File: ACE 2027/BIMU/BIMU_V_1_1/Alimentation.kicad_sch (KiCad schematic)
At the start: 16 parts, among them U101 AP7361C-33E

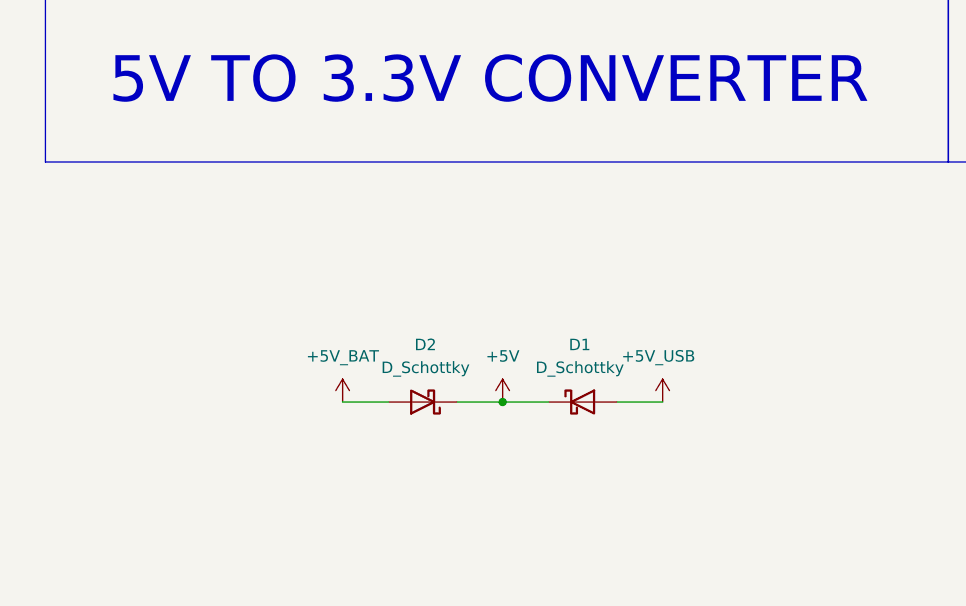
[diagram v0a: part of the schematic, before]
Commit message: Faire les modifications requise pour le pcb
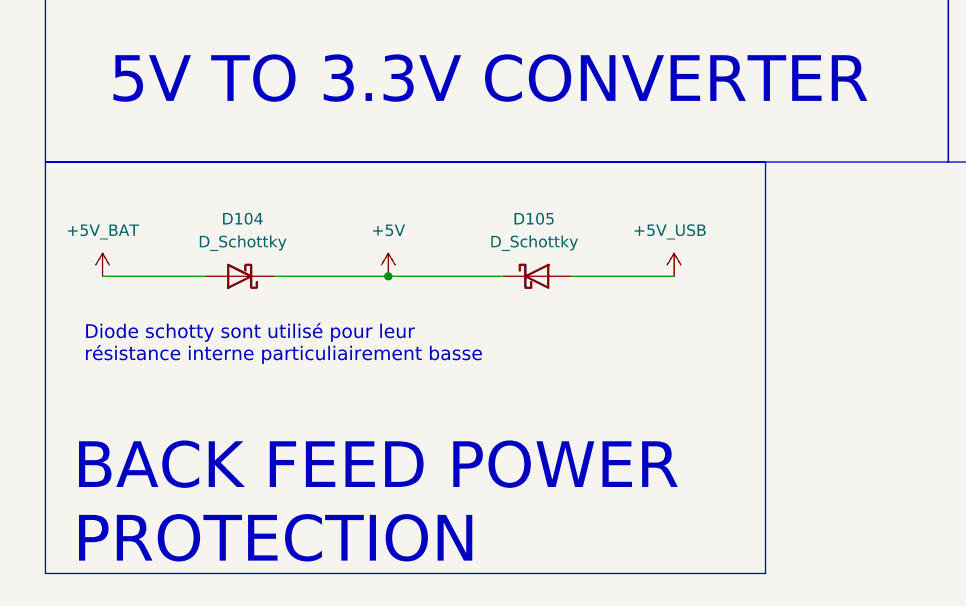
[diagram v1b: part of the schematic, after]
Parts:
- D104: renamed from D2; footprint Diode_SMD:D_3220_8050Metric_Pad2.65x5.15mm_HandSolder -> Diode_SMD:D_0805_2012Metric_Pad1.15x1.40mm_HandSolder
- D105: renamed from D1; footprint Diode_SMD:D_3220_8050Metric_Pad2.65x5.15mm_HandSolder -> Diode_SMD:D_0805_2012Metric_Pad1.15x1.40mm_HandSolder
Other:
- note added: "BACK FEED POWER PROTECTION"
- note added: "Diode schotty sont utilisé pour leur résistance interne particuliairement basse"
- moved on the sheet: D104, D105
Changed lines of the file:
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@@
+	)
+	(rectangle
+		(start 12.7 76.2)
+		(end 92.71 121.92)
+		(stroke
+			(width 0)
+			(type default)
+		)
+		(fill
+			(type none)
+		)
 	)
 	(rectangle
@@
 		(fill
 			(type none)
+		)
+	)
+	(text "Diode schotty sont utilisé pour leur \nrésistance interne particuliairement basse"
+		(exclude_from_sim no)
+		(at 17.018 96.52 0)
+		(effects
+			(font
+				(size 1.524 1.524)
+			)
+			(justify left)
+		)
+	)
+	(text "BACK FEED POWER\nPROTECTION"
+		(exclude_from_sim no)
+		(at 15.748 114.3 0)
+		(effects
+			(font
+				(size 5.08 5.08)
+			)
+			(justify left)
 		)
 	)
@@
 	)
 	(junction
-		(at 63.5 102.87)
+		(at 50.8 88.9)
 		(diameter 0)
 		(color 0 0 0 0)
@@
 	(wire
 		(pts
-			(xy 63.5 102.87) (xy 68.58 102.87)
+			(xy 50.8 88.9) (xy 63.5 88.9)
 		)
 		(stroke
@@
 	(wire
 		(pts
-			(xy 76.2 102.87) (xy 81.28 102.87)
+			(xy 71.12 88.9) (xy 82.55 88.9)
 		)
 		(stroke
@@
 	(wire
 		(pts
-			(xy 45.72 102.87) (xy 50.8 102.87)
-		)
-		(stroke
-			(width 0)
-			(type default)
-		)
-	)
-	(wire
-		(pts
-			(xy 58.42 102.87) (xy 63.5 102.87)
+			(xy 19.05 88.9) (xy 30.48 88.9)
+		)
+		(stroke
+			(width 0)
+			(type default)
+		)
+	)
+	(wire
+		(pts
+			(xy 38.1 88.9) (xy 50.8 88.9)
 		)
 		(stroke
@@
 	(symbol
 		(lib_id "power:+5V")
-		(at 45.72 102.87 0)
+		(at 19.05 88.9 0)
 		(unit 1)
 		(body_style 1)
@@
 		(dnp no)
 		(property "Reference" "#PWR0227"
-			(at 45.72 106.68 0)
+			(at 19.05 92.71 0)
 			(hide yes)
 			(show_name no)
@@
 		)
 		(property "Value" "+5V_BAT"
-			(at 45.72 97.79 0)
+			(at 19.05 83.82 0)
 			(show_name no)
 			(do_not_autoplace no)
@@
 		)
 		(property "Footprint" ""
-			(at 45.72 102.87 0)
+			(at 19.05 88.9 0)
 			(hide yes)
 			(show_name no)
@@
 		)
 		(property "Datasheet" ""
-			(at 45.72 102.87 0)
+			(at 19.05 88.9 0)
 			(hide yes)
 			(show_name no)
@@
 		)
 		(property "Description" "Power symbol creates a global label with name \"+5V\""
-			(at 45.72 102.87 0)
+			(at 19.05 88.9 0)
 			(hide yes)
 			(show_name no)
@@
 	(symbol
 		(lib_id "Device:D_Schottky")
-		(at 72.39 102.87 0)
+		(at 67.31 88.9 0)
 		(unit 1)
 		(body_style 1)
@@
 		(dnp no)
 		(fields_autoplaced yes)
-		(property "Reference" "D1"
-			(at 72.0725 96.52 0)
+		(property "Reference" "D105"
+			(at 66.9925 82.55 0)
 			(show_name no)
 			(do_not_autoplace no)
@@
 		)
 		(property "Value" "D_Schottky"
-			(at 72.0725 99.06 0)
-			(show_name no)
-			(do_not_autoplace no)
-			(effects
-				(font
-					(size 1.27 1.27)
-				)
-			)
-		)
-		(property "Footprint" "Diode_SMD:D_3220_8050Metric_Pad2.65x5.15mm_HandSolder"
-			(at 72.39 102.87 0)
+			(at 66.9925 85.09 0)
+			(show_name no)
+			(do_not_autoplace no)
+			(effects
+				(font
+					(size 1.27 1.27)
+				)
+			)
+		)
+		(property "Footprint" "Diode_SMD:D_0805_2012Metric_Pad1.15x1.40mm_HandSolder"
+			(at 67.31 88.9 0)
 			(hide yes)
 			(show_name no)
@@
 		)
 		(property "Datasheet" ""
-			(at 72.39 102.87 0)
+			(at 67.31 88.9 0)
 			(hide yes)
 			(show_name no)
@@
 		)
 		(property "Description" "Schottky diode"
-			(at 72.39 102.87 0)
+			(at 67.31 88.9 0)
 			(hide yes)
 			(show_name no)
@@
 		)
 		(property "Digi-Key_PN" "478-7800-1-ND"
-			(at 72.39 102.87 0)
+			(at 67.31 88.9 0)
 			(hide yes)
 			(show_name no)
@@
 			(project "BIMU_V_1_1"
 				(path "/abeb93ed-b9ef-4503-99a7-3fce380ff294/6937e765-eead-4ea7-ba07-6590a34338ab"
-					(reference "D1")
+					(reference "D105")
 					(unit 1)
 				)
@@
 	(symbol
 		(lib_id "power:+5V")
-		(at 81.28 102.87 0)
+		(at 82.55 88.9 0)
 		(unit 1)
 		(body_style 1)
@@
 		(dnp no)
 		(property "Reference" "#PWR0226"
-			(at 81.28 106.68 0)
+			(at 82.55 92.71 0)
 			(hide yes)
 			(show_name no)
@@
 		)
 		(property "Value" "+5V_USB"
-			(at 76.708 97.79 0)
+			(at 77.978 83.82 0)
 			(show_name no)
 			(do_not_autoplace no)
@@
 		)
 		(property "Footprint" ""
-			(at 81.28 102.87 0)
+			(at 82.55 88.9 0)
 			(hide yes)
 			(show_name no)
@@
 		)
 		(property "Datasheet" ""
-			(at 81.28 102.87 0)
+			(at 82.55 88.9 0)
 			(hide yes)
 			(show_name no)
@@
 		)
 		(property "Description" "Power symbol creates a global label with name \"+5V\""
-			(at 81.28 102.87 0)
+			(at 82.55 88.9 0)
 			(hide yes)
 			(show_name no)
@@
 	(symbol
 		(lib_id "power:+5V")
-		(at 63.5 102.87 0)
+		(at 50.8 88.9 0)
 		(unit 1)
 		(body_style 1)
@@
 		(fields_autoplaced yes)
 		(property "Reference" "#PWR0112"
-			(at 63.5 106.68 0)
+			(at 50.8 92.71 0)
 			(hide yes)
 			(show_name no)
@@
 		)
 		(property "Value" "+5V"
-			(at 63.5 97.79 0)
+			(at 50.8 83.82 0)
 			(show_name no)
 			(do_not_autoplace no)
@@
 		)
 		(property "Footprint" ""
-			(at 63.5 102.87 0)
+			(at 50.8 88.9 0)
 			(hide yes)
 			(show_name no)
@@
 		)
 		(property "Datasheet" ""
-			(at 63.5 102.87 0)
+			(at 50.8 88.9 0)
 			(hide yes)
 			(show_name no)
@@
 		)
 		(property "Description" "Power symbol creates a global label with name \"+5V\""
-			(at 63.5 102.87 0)
+			(at 50.8 88.9 0)
 			(hide yes)
 			(show_name no)
@@
 	(symbol
 		(lib_id "Device:D_Schottky")
-		(at 54.61 102.87 180)
+		(at 34.29 88.9 180)
 		(unit 1)
 		(body_style 1)
@@
 		(dnp no)
 		(fields_autoplaced yes)
-		(property "Reference" "D2"
-			(at 54.9275 96.52 0)
+		(property "Reference" "D104"
+			(at 34.6075 82.55 0)
 			(show_name no)
 			(do_not_autoplace no)
@@
 		)
 		(property "Value" "D_Schottky"
-			(at 54.9275 99.06 0)
-			(show_name no)
-			(do_not_autoplace no)
-			(effects
-				(font
-					(size 1.27 1.27)
-				)
-			)
-		)
-		(property "Footprint" "Diode_SMD:D_3220_8050Metric_Pad2.65x5.15mm_HandSolder"
-			(at 54.61 102.87 0)
+			(at 34.6075 85.09 0)
+			(show_name no)
+			(do_not_autoplace no)
+			(effects
+				(font
+					(size 1.27 1.27)
+				)
+			)
+		)
+		(property "Footprint" "Diode_SMD:D_0805_2012Metric_Pad1.15x1.40mm_HandSolder"
+			(at 34.29 88.9 0)
 			(hide yes)
 			(show_name no)
@@
 		)
 		(property "Datasheet" ""
-			(at 54.61 102.87 0)
+			(at 34.29 88.9 0)
 			(hide yes)
 			(show_name no)
@@
 		)
 		(property "Description" "Schottky diode"
-			(at 54.61 102.87 0)
+			(at 34.29 88.9 0)
 			(hide yes)
 			(show_name no)
@@
 		)
 		(property "Digi-Key_PN" "478-7800-1-ND"
-			(at 54.61 102.87 0)
+			(at 34.29 88.9 0)
 			(hide yes)
 			(show_name no)
@@
 			(project "BIMU_V_1_1"
 				(path "/abeb93ed-b9ef-4503-99a7-3fce380ff294/6937e765-eead-4ea7-ba07-6590a34338ab"
-					(reference "D2")
-					(unit 1)
-				)
+					(reference "D104")
+					(unit 1)
+				)
